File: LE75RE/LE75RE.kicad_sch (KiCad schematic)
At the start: 174 parts, among them P1 USB_C_Plug_USB2.0, SW1 SW_Push, U1 ATmega32U4-A, Y1 YSX321SL

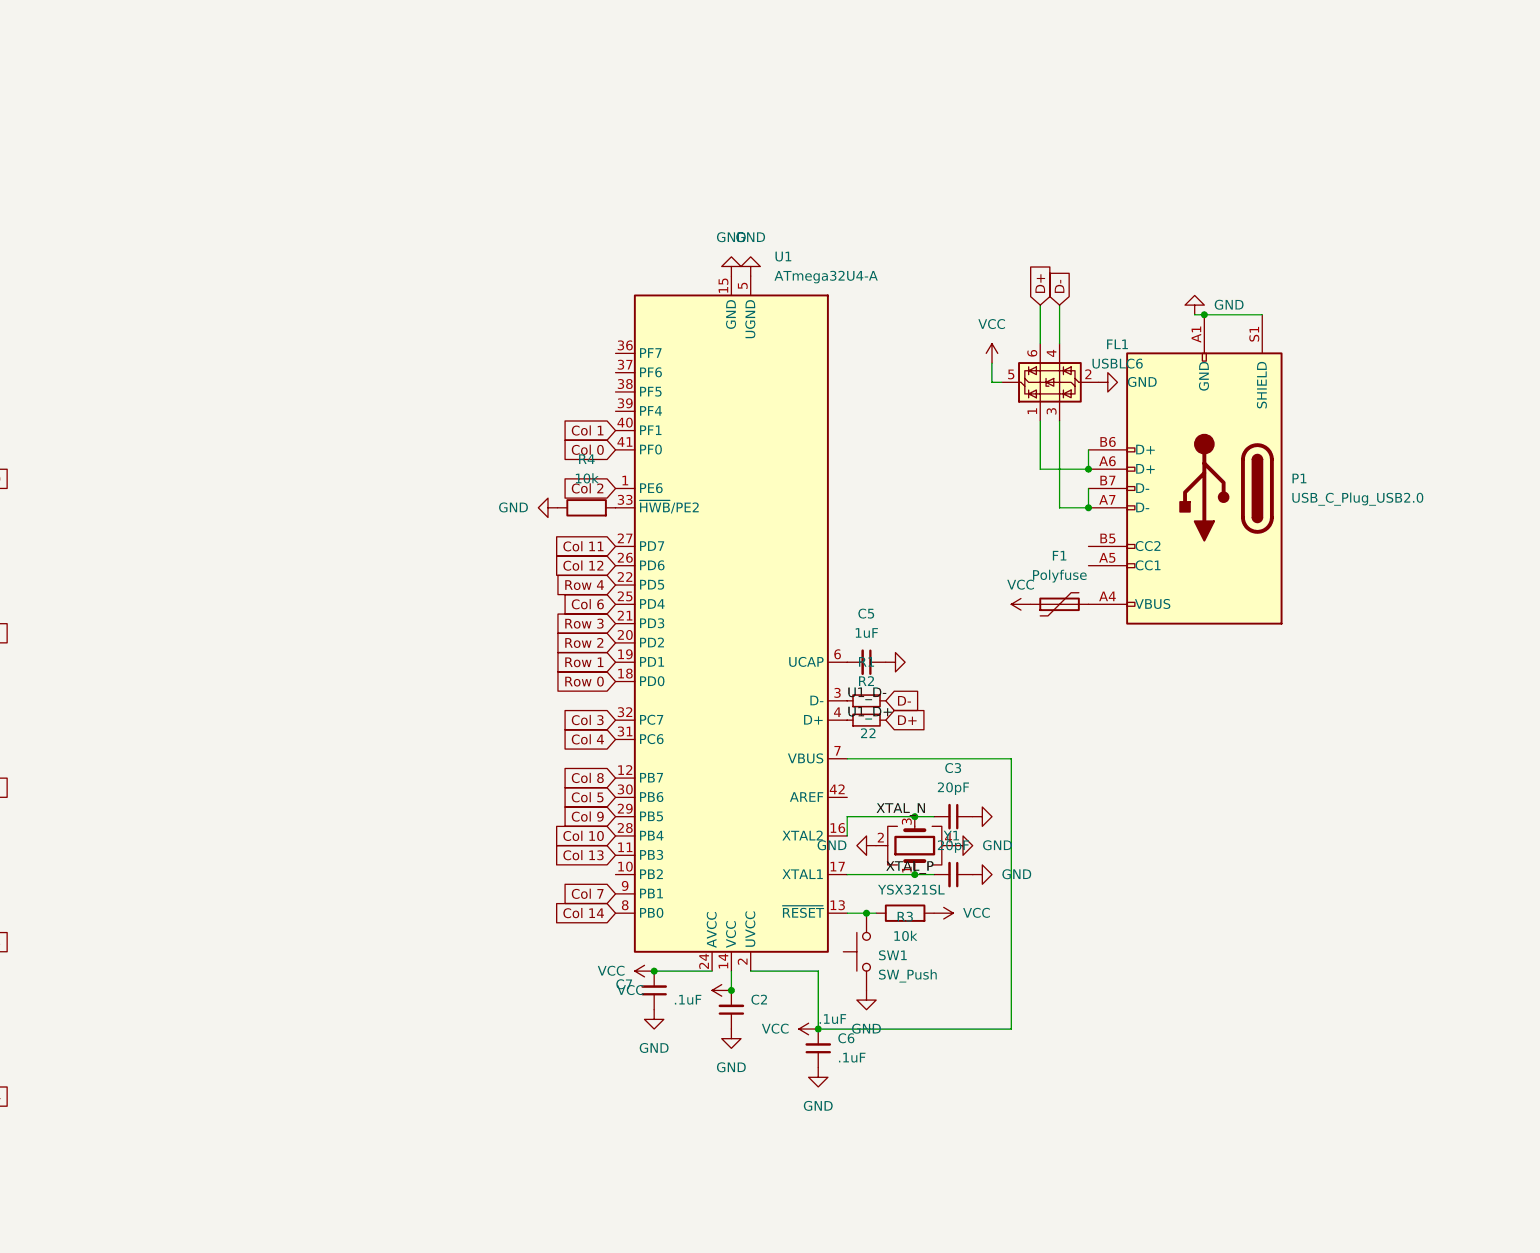
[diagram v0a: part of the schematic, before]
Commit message: Many changes
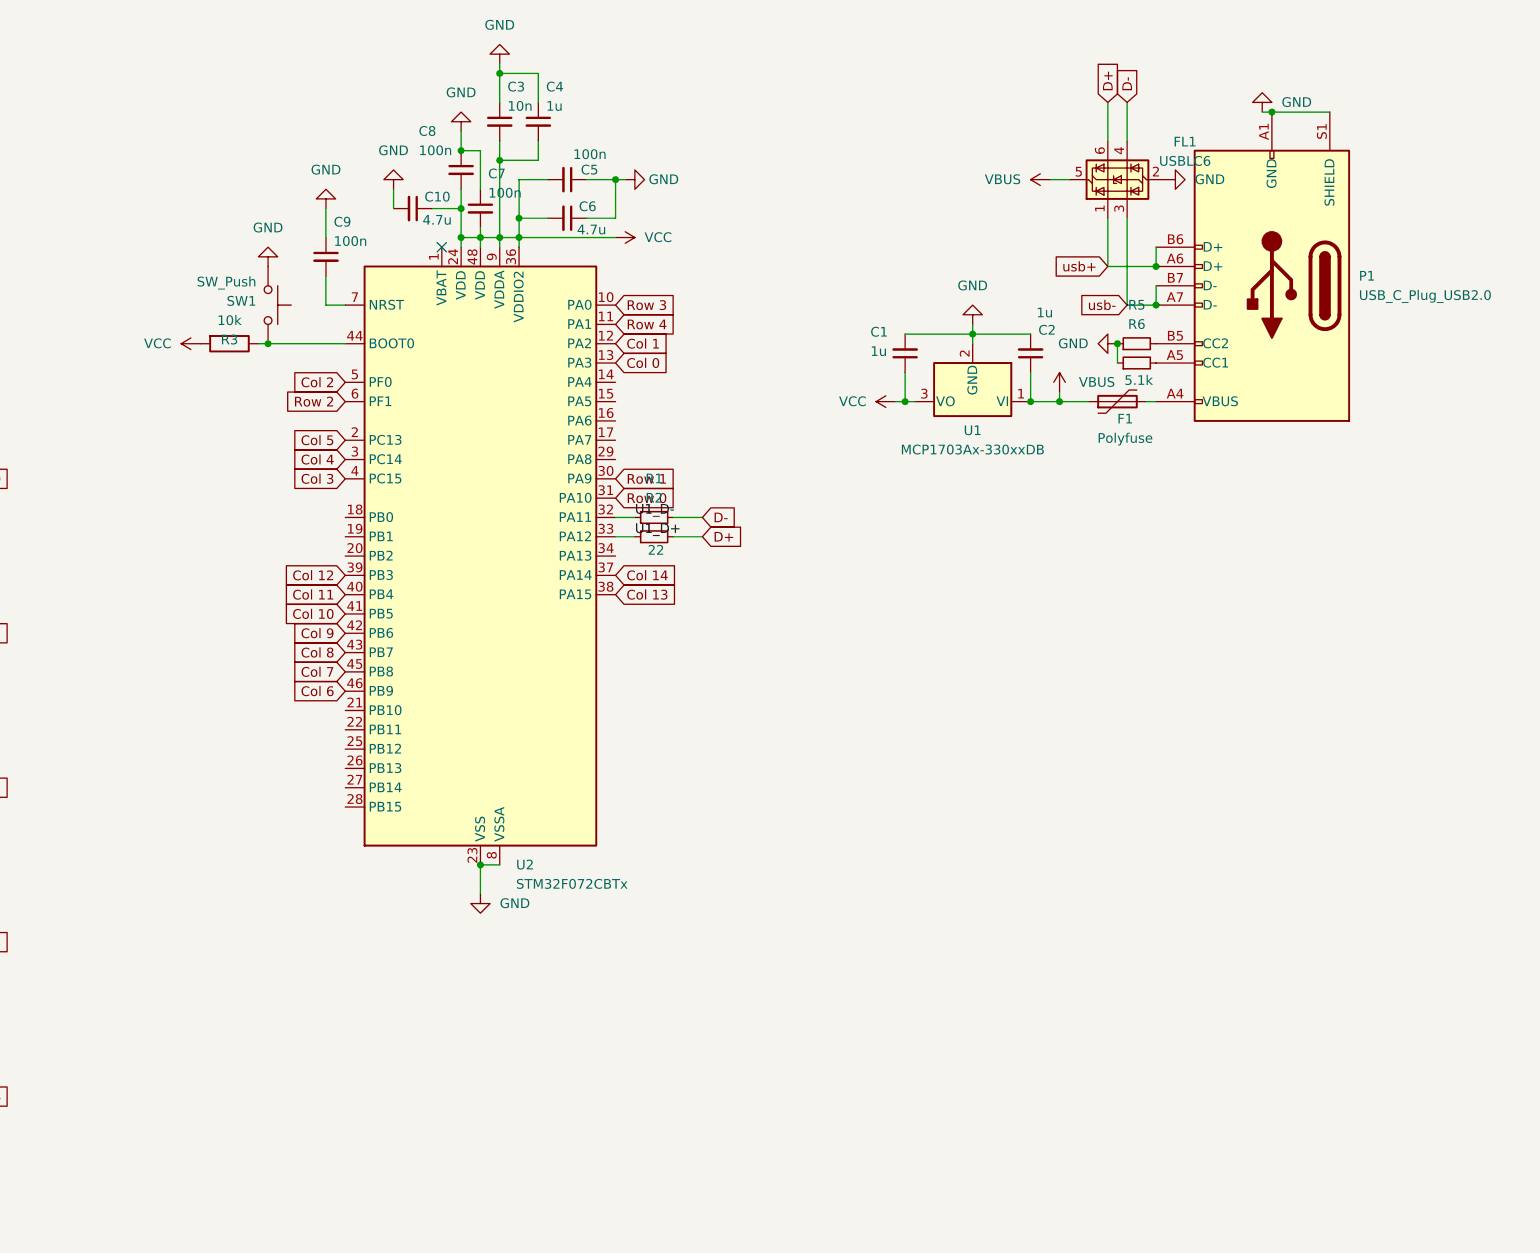
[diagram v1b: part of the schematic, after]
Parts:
- removed R4: 10k, Resistor_SMD:R_0603_1608Metric, symbol Device:R
- removed U1: ATmega32U4-A, Package_DFN_QFN:QFN-44-1EP_7x7mm_P0.5mm_EP5.2x5.2mm, symbol MCU_Microchip_ATmega:ATmega32U4-M
- removed Y1: YSX321SL, Crystal:Crystal_SMD_3225-4Pin_3.2x2.5mm, symbol Device:Crystal_GND24
- added C1: 1u, Capacitor_SMD:C_0603_1608Metric, symbol Device:C_Small
- added C10: 4.7u, Capacitor_SMD:C_0603_1608Metric, symbol Device:C_Small
- added C8, C9: 100n, Capacitor_SMD:C_0603_1608Metric, symbol Device:C_Small
- added R5, R6: 5.1k, Resistor_SMD:R_0603_1608Metric, symbol Device:R_Small
- added U1: MCP1703Ax-330xxDB, Package_TO_SOT_SMD:SOT-223-3_TabPin2, symbol Regulator_Linear:MCP1703Ax-330xxDB
- added U2: STM32F072CBTx, Package_QFP:LQFP-48_7x7mm_P0.5mm, symbol MCU_ST_STM32F0:STM32F072CBTx
- C2: value .1uF -> 1u
- C3: value 20pF -> 10n
- C4: value 20pF -> 1u
- C5: value 1uF -> 100n
- C6: value .1uF -> 4.7u
- C7: value .1uF -> 100n
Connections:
- net XTAL_N is gone; now on net VCC: C3.2
- net XTAL_P is gone; now on net VCC: C4.2
- net Col 0: now also U2.13 (PA3)
- net Col 1: now also U2.12 (PA2)
- net Col 10: now also U2.41 (PB5)
- net Col 11: now also U2.40 (PB4)
- net Col 12: now also U2.39 (PB3)
- net Col 13: now also U2.38 (PA15)
- net Col 14: now also U2.37 (PA14)
- net Col 2: now also U2.5 (PF0)
- net Col 3: now also U2.4 (PC15)
- net Col 4: now also U2.3 (PC14)
- net Col 5: now also U2.2 (PC13)
- net Col 6: now also U2.46 (PB9)
- net Col 7: now also U2.45 (PB8)
- net Col 8: now also U2.43 (PB7)
- net Col 9: now also U2.42 (PB6)
- net GND: now also C2.2, C1.2, C10.2, C8.1, C9.1, R5.1, R6.1, U1.2 (GND), U2.23 (VSS), U2.35 (VSS), U2.47 (VSS), U2.8 (VSSA); no longer C2.1
- net Row 0: now also U2.31 (PA10)
- net Row 1: now also U2.30 (PA9)
- net Row 2: now also U2.6 (PF1)
- net Row 3: now also U2.10 (PA0)
- net Row 4: now also U2.11 (PA1)
- net U1_D+: now also U2.33 (PA12)
- net U1_D-: now also U2.32 (PA11)
- net VCC: now also C5.2, C1.1, C10.1, C8.2, U1.3 (VO), U2.24 (VDD), U2.36 (VDDIO2), U2.48 (VDD), U2.9 (VDDA); no longer C2.2, F1.1, FL1.5 (VBUS)
- net usb+: now reaches FL1.1 (I/O1), P1.A6 (D+), P1.B6 (D+)
- net usb-: now reaches FL1.3 (I/O2), P1.A7 (D-), P1.B7 (D-)
- net at R3.1, SW1.2: now also U2.44 (BOOT0)
- net at P1.A5 (CC1): now also R6.2
- net at P1.B5 (CC2): now also R5.2
- new net: C9.2, U2.7 (NRST)
- new net VBUS: C2.1, F1.1, FL1.5 (VBUS), U1.1 (VI)
- no-connect marks 0 -> 1
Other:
- moved on the sheet: F1, FL1, P1, R1, R2, R3, SW1
